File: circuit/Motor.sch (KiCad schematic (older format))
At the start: 8 parts, among them J7 Conn_02x03_Odd_Even, J8 Conn_02x03_Odd_Even, U4 TB6612FNG

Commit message: Kicad v5.1.8対応
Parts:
- removed U4: TB6612FNG, Housings_SSOP:SSOP-24_5.3x8.2mm_Pitch0.65mm, symbol motor_drivers:TB6612FNG
- added U2: TB6612FNG, Package_SO:SSOP-24_5.3x8.2mm_P0.65mm, symbol Driver_Motor:TB6612FNG
- C16, C18: symbol device:CP -> Device:CP
- C17, C19, C20: symbol device:C -> Device:C
- J7, J8: symbol conn:Conn_02x03_Odd_Even -> Connector_Generic:Conn_02x03_Odd_Even
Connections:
- wire segments 75 -> 57
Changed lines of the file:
@@
 $EndDescr
-$Comp
-L motor_drivers:TB6612FNG U4
-U 1 1 5FA509D2
-P 4700 3800
-F 0 "U4" H 4700 4575 50  0000 C CNN
-F 1 "TB6612FNG" H 4700 4484 50  0000 C CNN
-F 2 "Housings_SSOP:SSOP-24_5.3x8.2mm_Pitch0.65mm" H 4700 4000 50  0001 C CNN
-F 3 "https://akizukidenshi.com/download/ds/Toshiba/TB6612FNG_datasheet_ja_20141001.pdf" H 4700 4000 50  0001 C CNN
-	1    4700 3800
-	1    0    0    -1
-$EndComp
 $Comp
 L power:VCC #PWR0136
@@
 $EndComp
 $Comp
-L device:CP C18
+L Device:CP C18
 U 1 1 5FA54BC5
 P 4150 2350
@@
 $EndComp
 $Comp
-L device:C C19
+L Device:C C19
 U 1 1 5FA556A7
 P 4600 2350
@@
 $EndComp
 $Comp
-L device:C C20
+L Device:C C20
 U 1 1 5FA55999
 P 5000 2350
@@
 L power:VCC #PWR0138
 U 1 1 5FA58843
-P 5400 3100
-F 0 "#PWR0138" H 5400 2950 50  0001 C CNN
-F 1 "VCC" H 5417 3273 50  0000 C CNN
-F 2 "" H 5400 3100 50  0001 C CNN
-F 3 "" H 5400 3100 50  0001 C CNN
-	1    5400 3100
+P 4950 3400
+F 0 "#PWR0138" H 4950 3250 50  0001 C CNN
+F 1 "VCC" H 4967 3573 50  0000 C CNN
+F 2 "" H 4950 3400 50  0001 C CNN
+F 3 "" H 4950 3400 50  0001 C CNN
+	1    4950 3400
 	1    0    0    -1
 $EndComp
@@
 	3150 2450 3150 2500
 $Comp
-L device:CP C16
+L Device:CP C16
 U 1 1 5FA5D47E
 P 3150 2300
@@
 $EndComp
 $Comp
-L device:C C17
+L Device:C C17
 U 1 1 5FA5F3FD
 P 3600 2300
@@
 Wire Wire Line
 	3600 2450 3600 2500
-Wire Wire Line
-	5400 3100 5400 3250
-Wire Wire Line
-	5400 3250 5300 3250
-Wire Wire Line
-	5400 3250 5400 4250
-Wire Wire Line
-	5400 4250 5300 4250
-Connection ~ 5400 3250
-Wire Wire Line
-	5400 4250 5400 4350
-Wire Wire Line
-	5400 4350 5300 4350
-Connection ~ 5400 4250
 $Comp
 L power:+3.3V #PWR0141
 U 1 1 5FA6429D
-P 5650 3100
-F 0 "#PWR0141" H 5650 2950 50  0001 C CNN
-F 1 "+3.3V" H 5665 3273 50  0000 C CNN
-F 2 "" H 5650 3100 50  0001 C CNN
-F 3 "" H 5650 3100 50  0001 C CNN
-	1    5650 3100
-	1    0    0    -1
-$EndComp
-Wire Wire Line
-	5650 3100 5650 3650
-Wire Wire Line
-	5650 3650 5300 3650
+P 4450 3400
+F 0 "#PWR0141" H 4450 3250 50  0001 C CNN
+F 1 "+3.3V" H 4465 3573 50  0000 C CNN
+F 2 "" H 4450 3400 50  0001 C CNN
+F 3 "" H 4450 3400 50  0001 C CNN
+	1    4450 3400
+	1    0    0    -1
+$EndComp
 $Comp
 L power:GND #PWR0142
 U 1 1 5FA64FCB
-P 5500 4550
-F 0 "#PWR0142" H 5500 4300 50  0001 C CNN
-F 1 "GND" H 5505 4377 50  0000 C CNN
-F 2 "" H 5500 4550 50  0001 C CNN
-F 3 "" H 5500 4550 50  0001 C CNN
-	1    5500 4550
-	1    0    0    -1
-$EndComp
-Wire Wire Line
-	5300 3850 5500 3850
-Wire Wire Line
-	5500 3850 5500 4550
+P 5050 5800
+F 0 "#PWR0142" H 5050 5550 50  0001 C CNN
+F 1 "GND" H 5055 5627 50  0000 C CNN
+F 2 "" H 5050 5800 50  0001 C CNN
+F 3 "" H 5050 5800 50  0001 C CNN
+	1    5050 5800
+	1    0    0    -1
+$EndComp
 $Comp
 L power:GND #PWR0143
 U 1 1 5FA66338
-P 3950 4600
-F 0 "#PWR0143" H 3950 4350 50  0001 C CNN
-F 1 "GND" H 3955 4427 50  0000 C CNN
-F 2 "" H 3950 4600 50  0001 C CNN
-F 3 "" H 3950 4600 50  0001 C CNN
-	1    3950 4600
-	1    0    0    -1
-$EndComp
-Wire Wire Line
-	4100 4150 3950 4150
-Wire Wire Line
-	3950 4150 3950 4600
-Wire Wire Line
-	4100 4050 3950 4050
-Wire Wire Line
-	3950 4050 3950 4150
-Connection ~ 3950 4150
-Wire Wire Line
-	4100 3550 3950 3550
-Wire Wire Line
-	3950 3550 3950 4050
-Connection ~ 3950 4050
-Wire Wire Line
-	4100 3450 3950 3450
-Wire Wire Line
-	3950 3450 3950 3550
-Connection ~ 3950 3550
-Text HLabel 6050 3350 2    50   Input ~ 0
+P 4450 5800
+F 0 "#PWR0143" H 4450 5550 50  0001 C CNN
+F 1 "GND" H 4455 5627 50  0000 C CNN
+F 2 "" H 4450 5800 50  0001 C CNN
+F 3 "" H 4450 5800 50  0001 C CNN
+	1    4450 5800
+	1    0    0    -1
+$EndComp
+Text HLabel 3950 4400 0    50   Input ~ 0
 PWM_L
-Wire Wire Line
-	5300 3350 6050 3350
-Text HLabel 6050 3450 2    50   Input ~ 0
+Text HLabel 3950 4800 0    50   Input ~ 0
 IN2_L
-Text HLabel 6050 3550 2    50   Input ~ 0
+Text HLabel 3950 4700 0    50   Input ~ 0
 IN1_L
-Wire Wire Line
-	5300 3450 6050 3450
-Wire Wire Line
-	5300 3550 6050 3550
-Text HLabel 6050 4150 2    50   Input ~ 0
+Text HLabel 3950 4500 0    50   Input ~ 0
 PWM_R
-Text HLabel 6050 3950 2    50   Input ~ 0
+Text HLabel 3950 4900 0    50   Input ~ 0
 IN1_R
-Text HLabel 6050 4050 2    50   Input ~ 0
+Text HLabel 3950 5000 0    50   Input ~ 0
 IN2_R
-Wire Wire Line
-	5300 3950 6050 3950
-Wire Wire Line
-	5300 4050 6050 4050
-Wire Wire Line
-	5300 4150 6050 4150
-Text HLabel 6050 3750 2    50   Input ~ 0
+Text HLabel 3950 4200 0    50   Input ~ 0
 STBY
-Wire Wire Line
-	5300 3750 6050 3750
-Wire Wire Line
-	3450 3250 3750 3250
-Wire Wire Line
-	4100 3350 3750 3350
-Wire Wire Line
-	3750 3350 3750 3250
-Connection ~ 3750 3250
-Wire Wire Line
-	3750 3250 4100 3250
-Wire Wire Line
-	3450 3650 3750 3650
-Wire Wire Line
-	3750 3650 4100 3650
-Wire Wire Line
-	4100 3750 3750 3750
-Wire Wire Line
-	3750 3750 3750 3650
-Connection ~ 3750 3650
-Wire Wire Line
-	3450 3850 3750 3850
-Wire Wire Line
-	4100 3950 3750 3950
-Wire Wire Line
-	3750 3950 3750 3850
-Connection ~ 3750 3850
-Wire Wire Line
-	3750 3850 4100 3850
-Wire Wire Line
-	3450 4250 3750 4250
-Wire Wire Line
-	4100 4350 3750 4350
-Wire Wire Line
-	3750 4350 3750 4250
-Connection ~ 3750 4250
-Wire Wire Line
-	3750 4250 4100 4250
-$Comp
-L conn:Conn_02x03_Odd_Even J7
+$Comp
+L Connector_Generic:Conn_02x03_Odd_Even J7
 U 1 1 5FA84090
 P 8050 3400
@@
 	8350 4800 8700 4800
 $Comp
-L conn:Conn_02x03_Odd_Even J8
+L Connector_Generic:Conn_02x03_Odd_Even J8
 U 1 1 5F9570AC
 P 8050 4700
@@
 	1    0    0    -1
 $EndComp
-Text Label 3450 3650 2    50   ~ 0
+Text Label 5450 4400 0    50   ~ 0
 MOTOR_L-
-Text Label 3450 3850 2    50   ~ 0
+Text Label 5450 4700 0    50   ~ 0
 MOTOR_R-
-Text Label 3450 4250 2    50   ~ 0
+Text Label 5450 4900 0    50   ~ 0
 MOTOR_R+
 Text Label 7500 3300 2    50   ~ 0
@@
 Text Label 8700 4600 0    50   ~ 0
 MOTOR_R-
-Text Label 3450 3250 2    50   ~ 0
+Text Label 5450 4200 0    50   ~ 0
 MOTOR_L+
+Wire Wire Line
+	4450 5600 4450 5800
+$Comp
+L Driver_Motor:TB6612FNG U2
+U 1 1 5FAE9218
+P 4750 4600
+F 0 "U2" H 4750 3511 50  0000 C CNN
+F 1 "TB6612FNG" H 4750 3420 50  0000 C CNN
+F 2 "Package_SO:SSOP-24_5.3x8.2mm_P0.65mm" H 6050 3700 50  0001 C CNN
+F 3 "https://toshiba.semicon-storage.com/us/product/linear/motordriver/detail.TB6612FNG.html" H 5200 5200 50  0001 C CNN
+	1    4750 4600
+	1    0    0    -1
+$EndComp
+Wire Wire Line
+	5350 4200 5450 4200
+Wire Wire Line
+	5350 4700 5450 4700
+Wire Wire Line
+	5350 4900 5450 4900
+Wire Wire Line
+	5350 4400 5450 4400
+Wire Wire Line
+	4850 5600 4850 5700
+Wire Wire Line
+	4850 5700 5050 5700
+Wire Wire Line
+	5050 5700 5050 5800
+Wire Wire Line
+	5050 5600 5050 5700
+Connection ~ 5050 5700
+Wire Wire Line
+	4950 3400 4950 3550
+Wire Wire Line
+	4850 3600 4850 3550
+Wire Wire Line
+	4850 3550 4950 3550
+Connection ~ 4950 3550
+Wire Wire Line
+	4950 3550 4950 3600
+Wire Wire Line
+	4950 3550 5050 3550
+Wire Wire Line
+	5050 3550 5050 3600
+Wire Wire Line
+	4450 3400 4450 3600
+Wire Wire Line
+	3950 4700 4150 4700
+Wire Wire Line
+	3950 4800 4150 4800
+Wire Wire Line
+	3950 4900 4150 4900
+Wire Wire Line
+	3950 5000 4150 5000
+Wire Wire Line
+	3950 4500 4150 4500
+Wire Wire Line
+	3950 4400 4150 4400
+Wire Wire Line
+	3950 4200 4150 4200
 $EndSCHEMATC

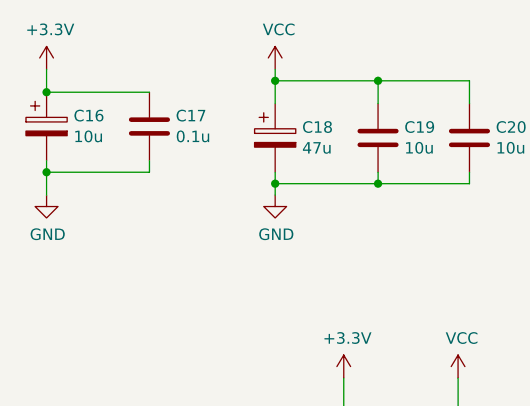
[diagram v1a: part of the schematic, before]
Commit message: Kicadのpcbnew映らないくてキレそう
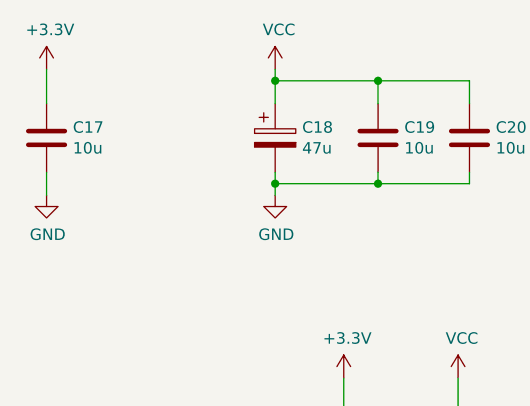
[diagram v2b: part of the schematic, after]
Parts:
- removed C16: 10u, symbol Device:CP
- C17: value 0.1u -> 10u; footprint (none) -> Capacitors_SMD:C_0805
- C18: footprint (none) -> Capacitors_SMD:CP_Elec_6.3x7.7
- C19, C20: footprint (none) -> Capacitors_SMD:C_0805
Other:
- moved on the sheet: C17
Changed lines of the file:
@@
 F 0 "C18" H 4268 2396 50  0000 L CNN
 F 1 "47u" H 4268 2305 50  0000 L CNN
-F 2 "" H 4188 2200 50  0001 C CNN
-F 3 "" H 4150 2350 50  0001 C CNN
+F 2 "Capacitors_SMD:CP_Elec_6.3x7.7" H 4600 1850 50  0001 C CNN
+F 3 "https://industrial.panasonic.com/cdbs/www-data/pdf/RDE0000/RDE0000COL98.pdf" H 4150 2350 50  0001 C CNN
 	1    4150 2350
 	1    0    0    -1
@@
 F 0 "C19" H 4715 2396 50  0000 L CNN
 F 1 "10u" H 4715 2305 50  0000 L CNN
-F 2 "" H 4638 2200 50  0001 C CNN
+F 2 "Capacitors_SMD:C_0805" H 4638 2200 50  0001 C CNN
 F 3 "" H 4600 2350 50  0001 C CNN
 	1    4600 2350
@@
 F 0 "C20" H 5115 2396 50  0000 L CNN
 F 1 "10u" H 5115 2305 50  0000 L CNN
-F 2 "" H 5038 2200 50  0001 C CNN
+F 2 "Capacitors_SMD:C_0805" H 5038 2200 50  0001 C CNN
 F 3 "" H 5000 2350 50  0001 C CNN
 	1    5000 2350
@@
 	1    0    0    -1
 $EndComp
-Wire Wire Line
-	3150 2050 3150 2150
-Wire Wire Line
-	3150 2450 3150 2500
-$Comp
-L Device:CP C16
-U 1 1 5FA5D47E
-P 3150 2300
-F 0 "C16" H 3268 2346 50  0000 L CNN
-F 1 "10u" H 3268 2255 50  0000 L CNN
-F 2 "" H 3188 2150 50  0001 C CNN
-F 3 "" H 3150 2300 50  0001 C CNN
-	1    3150 2300
-	1    0    0    -1
-$EndComp
 $Comp
 L Device:C C17
 U 1 1 5FA5F3FD
-P 3600 2300
-F 0 "C17" H 3715 2346 50  0000 L CNN
-F 1 "0.1u" H 3715 2255 50  0000 L CNN
-F 2 "" H 3638 2150 50  0001 C CNN
-F 3 "" H 3600 2300 50  0001 C CNN
-	1    3600 2300
-	1    0    0    -1
-$EndComp
-Wire Wire Line
-	3600 2500 3150 2500
-Connection ~ 3150 2500
-Wire Wire Line
-	3150 2500 3150 2600
-Wire Wire Line
-	3600 2150 3150 2150
-Connection ~ 3150 2150
-Wire Wire Line
-	3600 2450 3600 2500
+P 3150 2350
+F 0 "C17" H 3265 2396 50  0000 L CNN
+F 1 "10u" H 3265 2305 50  0000 L CNN
+F 2 "Capacitors_SMD:C_0805" H 3188 2200 50  0001 C CNN
+F 3 "" H 3150 2350 50  0001 C CNN
+	1    3150 2350
+	1    0    0    -1
+$EndComp
 $Comp
 L power:+3.3V #PWR0141
@@
 Wire Wire Line
 	3950 4200 4150 4200
+Wire Wire Line
+	3150 2050 3150 2200
+Wire Wire Line
+	3150 2500 3150 2600
 $EndSCHEMATC

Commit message: スーパーエンジニアの登竜門たる文彦は当然スーパーエンジニア
あってぃ許さない
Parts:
- C17, C19, C20: footprint Capacitors_SMD:C_0805 -> Capacitor_SMD:C_0805_2012Metric
- C18: footprint Capacitors_SMD:CP_Elec_6.3x7.7 -> Capacitor_SMD:CP_Elec_6.3x7.7
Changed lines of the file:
@@
 F 0 "C18" H 4268 2396 50  0000 L CNN
 F 1 "47u" H 4268 2305 50  0000 L CNN
-F 2 "Capacitors_SMD:CP_Elec_6.3x7.7" H 4600 1850 50  0001 C CNN
+F 2 "Capacitor_SMD:CP_Elec_6.3x7.7" H 4600 1850 50  0001 C CNN
 F 3 "https://industrial.panasonic.com/cdbs/www-data/pdf/RDE0000/RDE0000COL98.pdf" H 4150 2350 50  0001 C CNN
 	1    4150 2350
@@
 F 0 "C19" H 4715 2396 50  0000 L CNN
 F 1 "10u" H 4715 2305 50  0000 L CNN
-F 2 "Capacitors_SMD:C_0805" H 4638 2200 50  0001 C CNN
+F 2 "Capacitor_SMD:C_0805_2012Metric" H 4638 2200 50  0001 C CNN
 F 3 "" H 4600 2350 50  0001 C CNN
 	1    4600 2350
@@
 F 0 "C20" H 5115 2396 50  0000 L CNN
 F 1 "10u" H 5115 2305 50  0000 L CNN
-F 2 "Capacitors_SMD:C_0805" H 5038 2200 50  0001 C CNN
+F 2 "Capacitor_SMD:C_0805_2012Metric" H 5038 2200 50  0001 C CNN
 F 3 "" H 5000 2350 50  0001 C CNN
 	1    5000 2350
@@
 F 0 "C17" H 3265 2396 50  0000 L CNN
 F 1 "10u" H 3265 2305 50  0000 L CNN
-F 2 "Capacitors_SMD:C_0805" H 3188 2200 50  0001 C CNN
+F 2 "Capacitor_SMD:C_0805_2012Metric" H 3188 2200 50  0001 C CNN
 F 3 "" H 3150 2350 50  0001 C CNN
 	1    3150 2350
